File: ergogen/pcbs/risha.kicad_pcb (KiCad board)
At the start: 2 copper layers, 100 x 81 mm, 23 parts

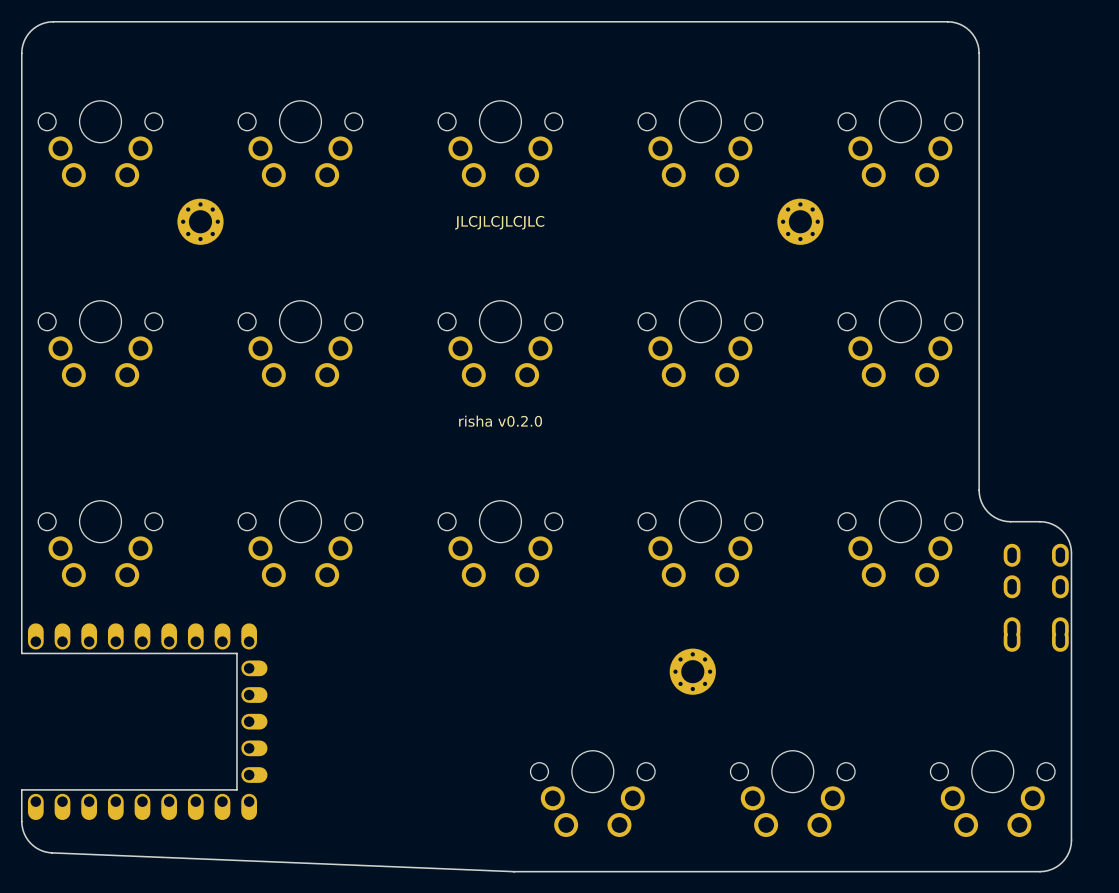
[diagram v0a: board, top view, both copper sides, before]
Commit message: converging on mx design
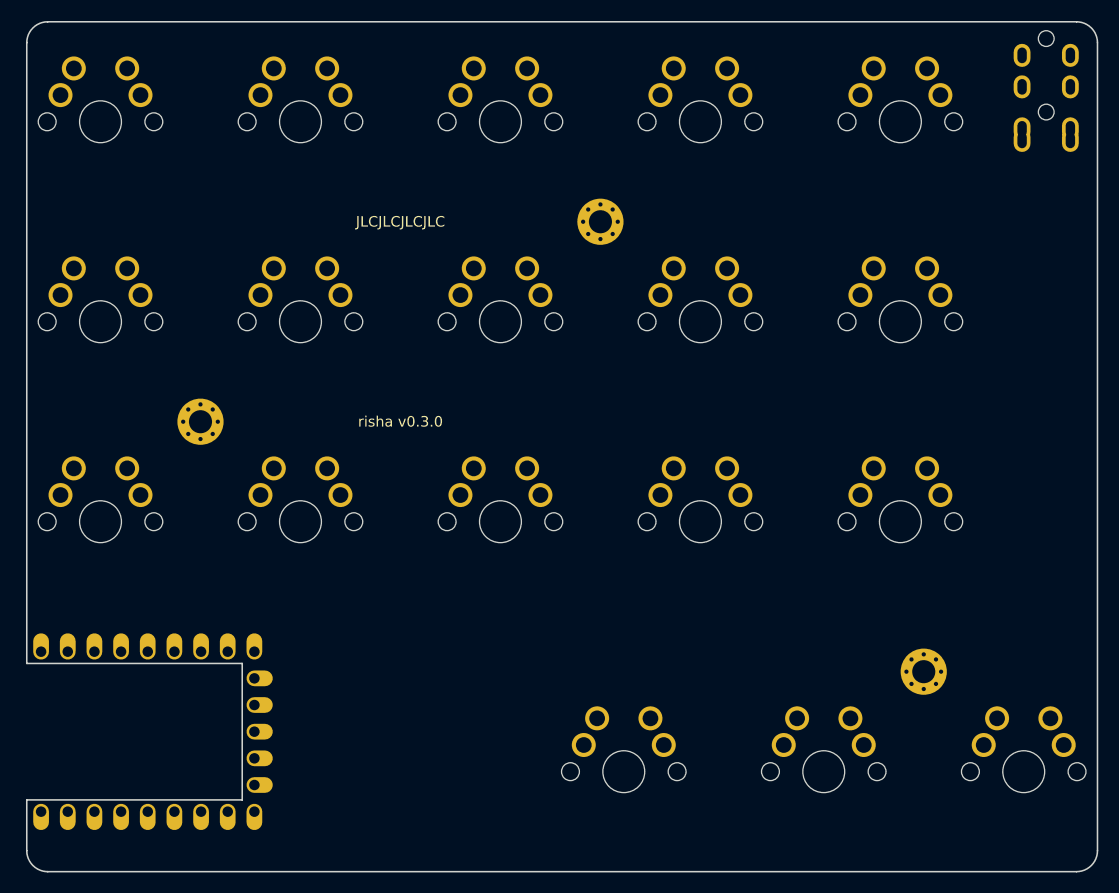
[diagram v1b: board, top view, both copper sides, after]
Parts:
- moved _4 52.6 mm to (161.9, 142.9)
- moved TRRS1 47.6 mm to (244.8, 104.8)
- moved _6 44.4 mm to (230.8, 166.7)
- moved _5 38.1 mm to (200.0, 123.8)
- moved S16 2.95 mm to (202.2, 176.2), turned to 0 degrees
- moved S17 2.95 mm to (221.3, 176.2), turned to 0 degrees
- moved S18 2.95 mm to (240.3, 176.2), turned to 0 degrees
- moved ? 1.08 mm to (156.9, 172.4)
- turned S1 to 0 degrees
- turned S10 to 0 degrees
- turned S11 to 0 degrees
- turned S12 to 0 degrees
- turned S13 to 0 degrees
- turned S14 to 0 degrees
- turned S15 to 0 degrees
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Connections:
- ? pad 1: matrix_pinky_bottom -> matrix_pinky_home
- ? pad 11: matrix_index_home -> matrix_index_bottom
- ? pad 12: matrix_index_bottom -> matrix_index_home
- ? pad 14: matrix_inner_top -> matrix_inner_home
- ? pad 15: matrix_inner_home -> matrix_inner_top
- ? pad 18: thumbfan_middle_home -> thumbfan_far_home
- ? pad 19: thumbfan_far_home -> thumbfan_middle_home
- ? pad 2: matrix_pinky_home -> matrix_pinky_bottom
- ? pad 4: matrix_ring_top -> matrix_ring_home
- ? pad 5: matrix_ring_home -> matrix_ring_top
- ? pad 7: matrix_middle_top -> matrix_middle_home
- ? pad 8: matrix_middle_home -> matrix_middle_bottom
- ? pad 9: matrix_middle_bottom -> matrix_middle_top
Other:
- board size 100 x 81 mm -> 102 x 81 mm
- board text added: "risha v0.3.0"
- board text removed: "risha v0.2.0"
